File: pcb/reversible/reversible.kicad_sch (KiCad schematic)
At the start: 83 parts, among them J1 PJ-320A, P1 OLED, SW1 Kailh hotswap MX socket, SW10 Kailh hotswap MX socket, SW11 Kailh hotswap MX socket, SW12 Kailh hotswap MX socket, SW13 Kailh hotswap MX socket, SW14 Kailh hotswap MX socket, SW15 Kailh hotswap MX socket, SW16 Kailh hotswap MX socket, SW17 Kailh hotswap MX socket, SW18 Kailh hotswap MX socket, SW19 Kailh hotswap MX socket, SW2 Kailh hotswap MX socket, SW20 Kailh hotswap MX socket, SW21 Kailh hotswap MX socket, SW22 Kailh hotswap MX socket, SW23 Kailh hotswap MX socket, SW24 Kailh hotswap MX socket, SW25 Kailh hotswap MX socket, SW26 Kailh hotswap MX socket, SW27 Kailh hotswap MX socket, SW28 Kailh hotswap MX socket, SW29 Kailh hotswap MX socket, SW3 Kailh hotswap MX socket, SW4 Kailh hotswap MX socket, SW5 Kailh hotswap MX socket, SW6 Kailh hotswap MX socket, SW7 Kailh hotswap MX socket, SW8 Kailh hotswap MX socket, SW9 Kailh hotswap MX socket, U1 ProMicro

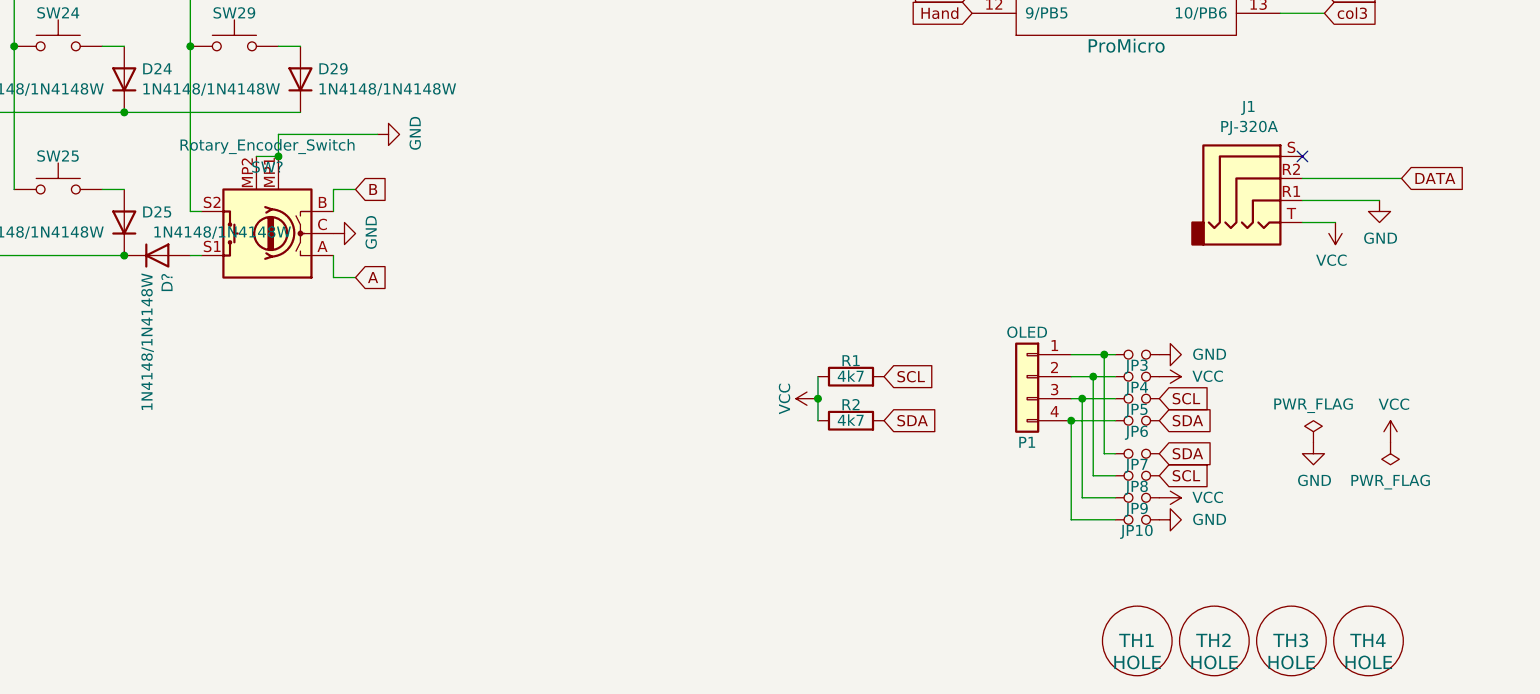
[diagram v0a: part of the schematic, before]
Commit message: layout designed
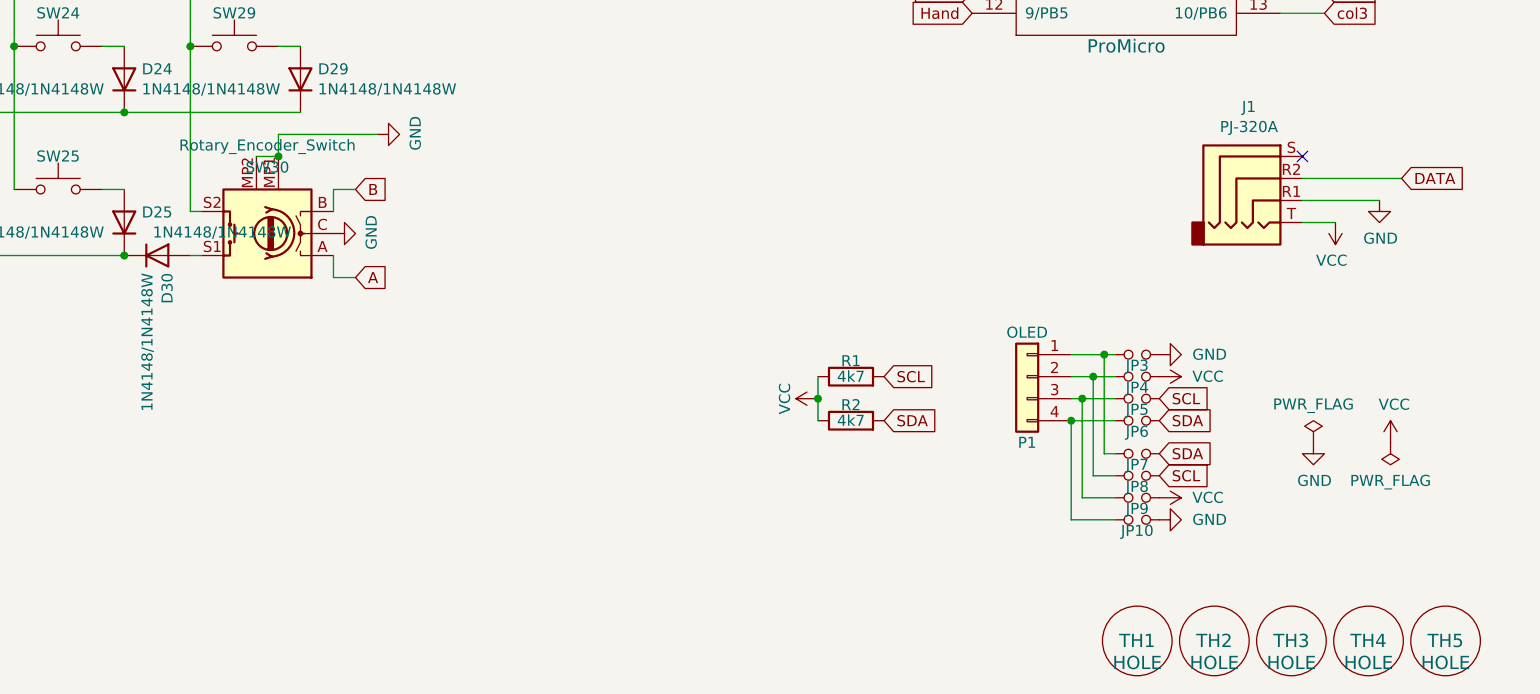
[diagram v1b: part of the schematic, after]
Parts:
- added TH5: HOLE, MountingHole:MountingHole_3.7mm, symbol keebio:Hole
- D30: renamed from D?; footprint Keyboard Library:Diode_DO35_SOD123 -> lowProfile:Diode_TH_SOD123
- SW30: renamed from SW?; footprint Keyboard Library:RotaryEncoder_Alps_EC11E-Switch_Vertical_H20_special -> lowProfile:RotaryEncoder_Alps_EC12E-Switch_Vertical_H20mm
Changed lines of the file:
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@@
 		(on_board yes)
 		(dnp no)
-		(property "Reference" "SW?"
+		(property "Reference" "SW30"
 			(at 139.7 97.79 0)
 			(effects
@@
 			)
 		)
-		(property "Footprint" "Keyboard Library:RotaryEncoder_Alps_EC11E-Switch_Vertical_H20_special"
+		(property "Footprint" "lowProfile:RotaryEncoder_Alps_EC12E-Switch_Vertical_H20mm"
 			(at 143.51 109.474 0)
 			(effects
@@
 			(project "reversible"
 				(path "/4b5512f1-4036-44b1-a4c2-dbd3b8563587"
-					(reference "SW?")
+					(reference "SW30")
 					(unit 1)
 				)
@@
 	)
 	(symbol
+		(lib_id "keebio:Hole")
+		(at 275.59 152.4 0)
+		(unit 1)
+		(exclude_from_sim no)
+		(in_bom yes)
+		(on_board yes)
+		(dnp no)
+		(property "Reference" "TH5"
+			(at 275.59 152.4 0)
+			(effects
+				(font
+					(size 1.524 1.524)
+				)
+			)
+		)
+		(property "Value" "HOLE"
+			(at 275.59 154.94 0)
+			(effects
+				(font
+					(size 1.524 1.524)
+				)
+			)
+		)
+		(property "Footprint" "MountingHole:MountingHole_3.7mm"
+			(at 275.59 152.4 0)
+			(effects
+				(font
+					(size 1.524 1.524)
+				)
+				(hide yes)
+			)
+		)
+		(property "Datasheet" ""
+			(at 275.59 152.4 0)
+			(effects
+				(font
+					(size 1.524 1.524)
+				)
+			)
+		)
+		(property "Description" ""
+			(at 275.59 152.4 0)
+			(effects
+				(font
+					(size 1.27 1.27)
+				)
+				(hide yes)
+			)
+		)
+		(instances
+			(project "reversible"
+				(path "/4b5512f1-4036-44b1-a4c2-dbd3b8563587"
+					(reference "TH5")
+					(unit 1)
+				)
+			)
+		)
+	)
+	(symbol
 		(lib_id "Device:D")
 		(at 82.55 38.1 90)
@@
 		(on_board yes)
 		(dnp no)
-		(property "Reference" "D?"
+		(property "Reference" "D30"
 			(at 128.1684 109.9566 90)
 			(effects
@@
 			)
 		)
-		(property "Footprint" "Keyboard Library:Diode_DO35_SOD123"
+		(property "Footprint" "lowProfile:Diode_TH_SOD123"
 			(at 127 107.95 0)
 			(effects
@@
 			(project "reversible"
 				(path "/4b5512f1-4036-44b1-a4c2-dbd3b8563587"
-					(reference "D?")
+					(reference "D30")
 					(unit 1)
 				)
